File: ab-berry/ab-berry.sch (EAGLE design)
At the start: 27 parts, among them U1 LM1117MPX-3.3/NOPB or AP2114H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

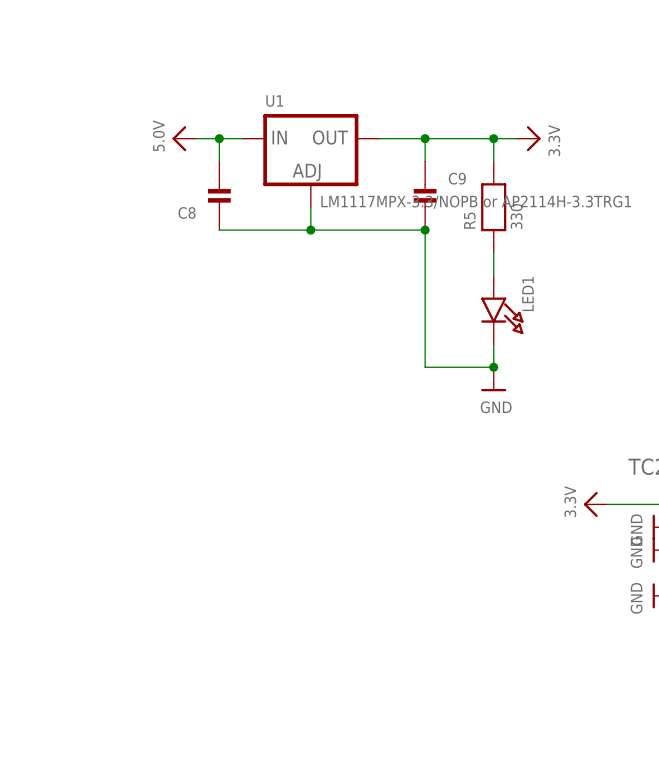
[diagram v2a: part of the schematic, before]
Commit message: wip
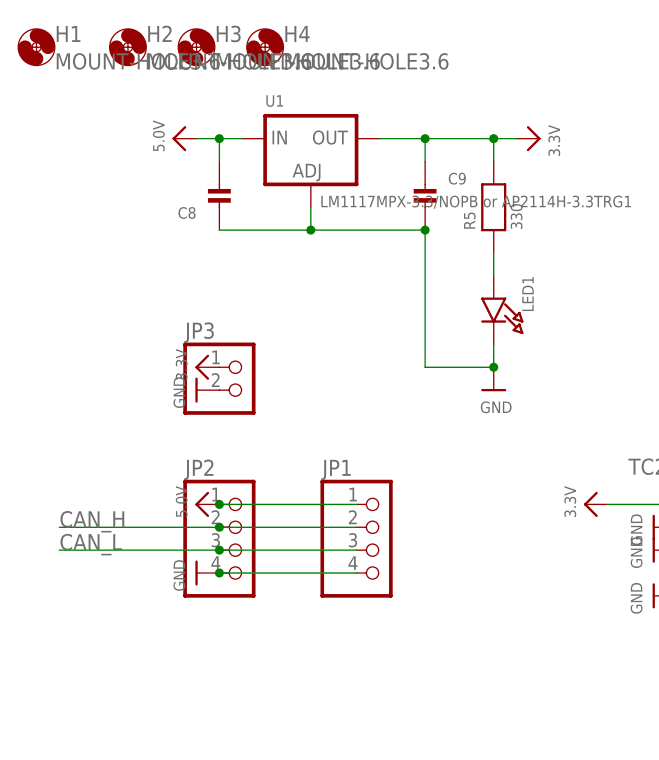
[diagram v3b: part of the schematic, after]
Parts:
- added H1, H2, H3, H4: MOUNT-HOLE3.6, holes:MOUNT-HOLE3.6
- added JP1, JP2: (no value), keves:PINHD-1X4
- added JP3: (no value), pinhead:PINHD-1X2
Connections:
- net 3.3V: now also JP3.1
- net 5.0V: now also JP1.1, JP2.1
- net CAN_H: now also JP1.2, JP2.2
- net CAN_L: now also JP1.3, JP2.3
- net GND: now also JP1.4, JP2.4, JP3.2
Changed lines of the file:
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@@
 <part name="U$27" library="microbuilder" deviceset="GND" device=""/>
 <part name="U$28" library="microbuilder" deviceset="3.3V" device=""/>
+<part name="JP1" library="keves" deviceset="PINHD-1X4" device=""/>
+<part name="JP2" library="keves" deviceset="PINHD-1X4" device=""/>
+<part name="U$30" library="microbuilder" deviceset="GND" device=""/>
+<part name="H1" library="holes" deviceset="MOUNT-HOLE" device="3.6"/>
+<part name="H2" library="holes" deviceset="MOUNT-HOLE" device="3.6"/>
+<part name="H3" library="holes" deviceset="MOUNT-HOLE" device="3.6"/>
+<part name="H4" library="holes" deviceset="MOUNT-HOLE" device="3.6"/>
+<part name="U$29" library="microbuilder" deviceset="5.0V" device=""/>
+<part name="JP3" library="pinhead" deviceset="PINHD-1X2" device=""/>
+<part name="U$31" library="microbuilder" deviceset="3.3V" device=""/>
+<part name="U$32" library="microbuilder" deviceset="GND" device=""/>
 </parts>
 <sheets>
@@
 <instance part="U$27" gate="G$1" x="109.22" y="-53.34" rot="R270"/>
 <instance part="U$28" gate="G$1" x="109.22" y="-50.8" rot="R90"/>
+<instance part="JP1" gate="A" x="-50.8" y="38.1"/>
+<instance part="JP2" gate="A" x="-66.04" y="38.1"/>
+<instance part="U$30" gate="G$1" x="-71.12" y="35.56" rot="R270"/>
+<instance part="H1" gate="G$1" x="-88.9" y="93.98"/>
+<instance part="H2" gate="G$1" x="-78.74" y="93.98"/>
+<instance part="H3" gate="G$1" x="-71.12" y="93.98"/>
+<instance part="H4" gate="G$1" x="-63.5" y="93.98"/>
+<instance part="U$29" gate="G$1" x="-71.12" y="43.18" rot="R90"/>
+<instance part="JP3" gate="G$1" x="-66.04" y="55.88"/>
+<instance part="U$31" gate="G$1" x="-71.12" y="58.42" rot="R90"/>
+<instance part="U$32" gate="G$1" x="-71.12" y="55.88" rot="R270"/>
 </instances>
 <busses>
@@
 <pinref part="LCD2" gate="G$1" pin="GND"/>
 <pinref part="U$27" gate="G$1" pin="GND"/>
+</segment>
+<segment>
+<pinref part="JP1" gate="A" pin="4"/>
+<pinref part="JP2" gate="A" pin="4"/>
+<wire x1="-68.58" y1="35.56" x2="-53.34" y2="35.56" width="0.1524" layer="91"/>
+<pinref part="U$30" gate="G$1" pin="GND"/>
+<junction x="-68.58" y="35.56"/>
+</segment>
+<segment>
+<pinref part="JP3" gate="G$1" pin="2"/>
+<pinref part="U$32" gate="G$1" pin="GND"/>
 </segment>
 </net>
@@
 <junction x="111.76" y="-50.8"/>
 </segment>
+<segment>
+<pinref part="JP3" gate="G$1" pin="1"/>
+<pinref part="U$31" gate="G$1" pin="3.3V"/>
+</segment>
 </net>
 <net name="SWDIO" class="0">
@@
 <label x="55.88" y="-22.86" size="1.778" layer="95"/>
 </segment>
+<segment>
+<pinref part="JP1" gate="A" pin="2"/>
+<pinref part="JP2" gate="A" pin="2"/>
+<wire x1="-68.58" y1="40.64" x2="-53.34" y2="40.64" width="0.1524" layer="91"/>
+<wire x1="-68.58" y1="40.64" x2="-86.36" y2="40.64" width="0.1524" layer="91"/>
+<junction x="-68.58" y="40.64"/>
+<label x="-86.36" y="40.64" size="1.778" layer="95"/>
+</segment>
 </net>
 <net name="CAN_L" class="0">
@@
 <wire x1="50.8" y1="-27.94" x2="58.42" y2="-27.94" width="0.1524" layer="91"/>
 <label x="55.88" y="-27.94" size="1.778" layer="95"/>
+</segment>
+<segment>
+<pinref part="JP1" gate="A" pin="3"/>
+<pinref part="JP2" gate="A" pin="3"/>
+<wire x1="-68.58" y1="38.1" x2="-53.34" y2="38.1" width="0.1524" layer="91"/>
+<wire x1="-68.58" y1="38.1" x2="-86.36" y2="38.1" width="0.1524" layer="91"/>
+<junction x="-68.58" y="38.1"/>
+<label x="-86.36" y="38.1" size="1.778" layer="95"/>
 </segment>
 </net>
@@
 <junction x="-68.58" y="83.82"/>
 </segment>
-</net>
+<segment>
+<pinref part="JP1" gate="A" pin="1"/>
+<pinref part="JP2" gate="A" pin="1"/>
+<wire x1="-68.58" y1="43.18" x2="-53.34" y2="43.18" width="0.1524" layer="91"/>
+<pinref part="U$29" gate="G$1" pin="5.0V"/>
+<junction x="-68.58" y="43.18"/>
+</segment>
+</net>

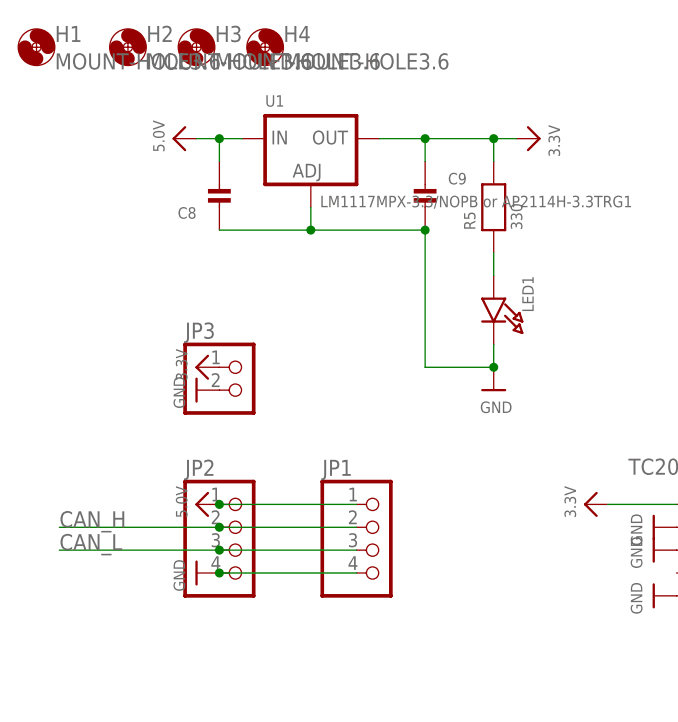
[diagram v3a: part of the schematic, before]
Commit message: wip
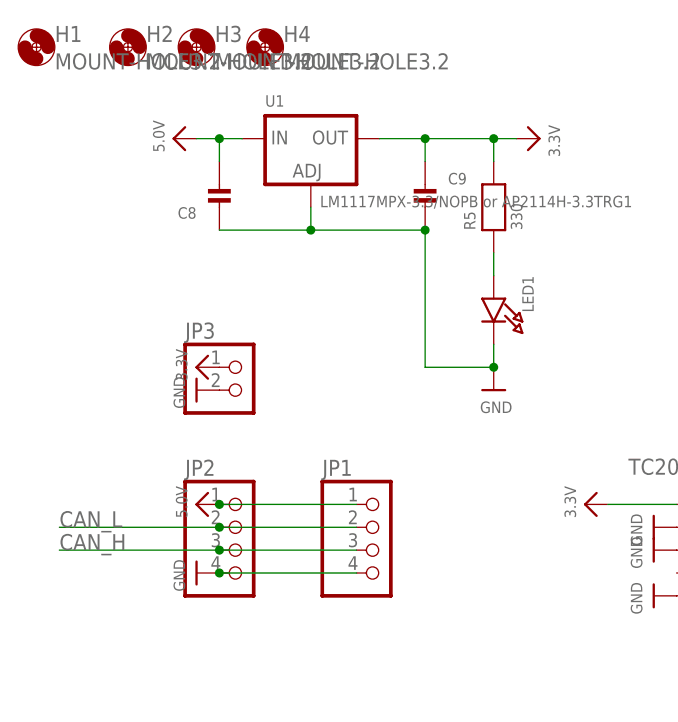
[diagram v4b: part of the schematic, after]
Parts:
- H1, H2, H3, H4: value MOUNT-HOLE3.6 -> MOUNT-HOLE3.2; device holes:MOUNT-HOLE3.6 -> holes:MOUNT-HOLE3.2
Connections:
- net CAN_H: now also JP1.3, JP2.3; no longer JP1.2, JP2.2
- net CAN_L: now also JP1.2, JP2.2; no longer JP1.3, JP2.3
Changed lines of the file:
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@@
 <grid distance="0.1" unitdist="inch" unit="inch" style="lines" multiple="1" display="no" altdistance="0.01" altunitdist="inch" altunit="inch"/>
 <layers>
-<layer number="1" name="Top" color="4" fill="1" visible="no" active="no"/>
-<layer number="16" name="Bottom" color="1" fill="1" visible="no" active="no"/>
-<layer number="17" name="Pads" color="2" fill="1" visible="no" active="no"/>
-<layer number="18" name="Vias" color="2" fill="1" visible="no" active="no"/>
-<layer number="19" name="Unrouted" color="6" fill="1" visible="no" active="no"/>
-<layer number="20" name="Dimension" color="15" fill="1" visible="no" active="no"/>
-<layer number="21" name="tPlace" color="7" fill="1" visible="no" active="no"/>
-<layer number="22" name="bPlace" color="7" fill="1" visible="no" active="no"/>
-<layer number="23" name="tOrigins" color="15" fill="1" visible="no" active="no"/>
-<layer number="24" name="bOrigins" color="15" fill="1" visible="no" active="no"/>
-<layer number="25" name="tNames" color="7" fill="1" visible="no" active="no"/>
-<layer number="26" name="bNames" color="7" fill="1" visible="no" active="no"/>
-<layer number="27" name="tValues" color="7" fill="1" visible="no" active="no"/>
-<layer number="28" name="bValues" color="7" fill="1" visible="no" active="no"/>
+<layer number="1" name="Top" color="4" fill="1" visible="yes" active="no"/>
+<layer number="16" name="Bottom" color="1" fill="1" visible="yes" active="no"/>
+<layer number="17" name="Pads" color="2" fill="1" visible="yes" active="no"/>
+<layer number="18" name="Vias" color="2" fill="1" visible="yes" active="no"/>
+<layer number="19" name="Unrouted" color="6" fill="1" visible="yes" active="no"/>
+<layer number="20" name="Dimension" color="15" fill="1" visible="yes" active="no"/>
+<layer number="21" name="tPlace" color="7" fill="1" visible="yes" active="no"/>
+<layer number="22" name="bPlace" color="7" fill="1" visible="yes" active="no"/>
+<layer number="23" name="tOrigins" color="15" fill="1" visible="yes" active="no"/>
+<layer number="24" name="bOrigins" color="15" fill="1" visible="yes" active="no"/>
+<layer number="25" name="tNames" color="7" fill="1" visible="yes" active="no"/>
+<layer number="26" name="bNames" color="7" fill="1" visible="yes" active="no"/>
+<layer number="27" name="tValues" color="7" fill="1" visible="yes" active="no"/>
+<layer number="28" name="bValues" color="7" fill="1" visible="yes" active="no"/>
 <layer number="29" name="tStop" color="7" fill="3" visible="no" active="no"/>
 <layer number="30" name="bStop" color="7" fill="6" visible="no" active="no"/>
@@
 <layer number="35" name="tGlue" color="7" fill="4" visible="no" active="no"/>
 <layer number="36" name="bGlue" color="7" fill="5" visible="no" active="no"/>
-<layer number="37" name="tTest" color="7" fill="1" visible="no" active="no"/>
-<layer number="38" name="bTest" color="7" fill="1" visible="no" active="no"/>
+<layer number="37" name="tTest" color="7" fill="1" visible="yes" active="no"/>
+<layer number="38" name="bTest" color="7" fill="1" visible="yes" active="no"/>
 <layer number="39" name="tKeepout" color="4" fill="11" visible="no" active="no"/>
 <layer number="40" name="bKeepout" color="1" fill="11" visible="no" active="no"/>
@@
 <layer number="44" name="Drills" color="7" fill="1" visible="no" active="no"/>
 <layer number="45" name="Holes" color="7" fill="1" visible="no" active="no"/>
-<layer number="46" name="Milling" color="3" fill="1" visible="no" active="no"/>
-<layer number="47" name="Measures" color="7" fill="1" visible="no" active="no"/>
-<layer number="48" name="Document" color="7" fill="1" visible="no" active="no"/>
-<layer number="49" name="Reference" color="7" fill="1" visible="no" active="no"/>
-<layer number="50" name="dxf" color="7" fill="1" visible="no" active="no"/>
-<layer number="51" name="tDocu" color="7" fill="1" visible="no" active="no"/>
-<layer number="52" name="bDocu" color="7" fill="1" visible="no" active="no"/>
-<layer number="53" name="tGND_GNDA" color="7" fill="9" visible="no" active="no"/>
-<layer number="54" name="bGND_GNDA" color="1" fill="9" visible="no" active="no"/>
-<layer number="56" name="wert" color="7" fill="1" visible="no" active="no"/>
+<layer number="46" name="Milling" color="3" fill="1" visible="yes" active="no"/>
+<layer number="47" name="Measures" color="7" fill="1" visible="yes" active="no"/>
+<layer number="48" name="Document" color="7" fill="1" visible="yes" active="no"/>
+<layer number="49" name="Reference" color="7" fill="1" visible="yes" active="no"/>
+<layer number="50" name="dxf" color="7" fill="1" visible="yes" active="no"/>
+<layer number="51" name="tDocu" color="7" fill="1" visible="yes" active="no"/>
+<layer number="52" name="bDocu" color="7" fill="1" visible="yes" active="no"/>
+<layer number="53" name="tGND_GNDA" color="7" fill="9" visible="yes" active="no"/>
+<layer number="54" name="bGND_GNDA" color="1" fill="9" visible="yes" active="no"/>
+<layer number="56" name="wert" color="7" fill="1" visible="yes" active="no"/>
 <layer number="90" name="Modules" color="5" fill="1" visible="yes" active="yes"/>
 <layer number="91" name="Nets" color="2" fill="1" visible="yes" active="yes"/>
@@
 <part name="JP2" library="keves" deviceset="PINHD-1X4" device=""/>
 <part name="U$30" library="microbuilder" deviceset="GND" device=""/>
-<part name="H1" library="holes" deviceset="MOUNT-HOLE" device="3.6"/>
-<part name="H2" library="holes" deviceset="MOUNT-HOLE" device="3.6"/>
-<part name="H3" library="holes" deviceset="MOUNT-HOLE" device="3.6"/>
-<part name="H4" library="holes" deviceset="MOUNT-HOLE" device="3.6"/>
+<part name="H1" library="holes" deviceset="MOUNT-HOLE" device="3.2" value="MOUNT-HOLE3.2"/>
+<part name="H2" library="holes" deviceset="MOUNT-HOLE" device="3.2" value="MOUNT-HOLE3.2"/>
+<part name="H3" library="holes" deviceset="MOUNT-HOLE" device="3.2" value="MOUNT-HOLE3.2"/>
+<part name="H4" library="holes" deviceset="MOUNT-HOLE" device="3.2" value="MOUNT-HOLE3.2"/>
 <part name="U$29" library="microbuilder" deviceset="5.0V" device=""/>
 <part name="JP3" library="pinhead" deviceset="PINHD-1X2" device=""/>
@@
 </segment>
 <segment>
+<pinref part="JP1" gate="A" pin="3"/>
+<pinref part="JP2" gate="A" pin="3"/>
+<wire x1="-68.58" y1="38.1" x2="-53.34" y2="38.1" width="0.1524" layer="91"/>
+<wire x1="-68.58" y1="38.1" x2="-86.36" y2="38.1" width="0.1524" layer="91"/>
+<junction x="-68.58" y="38.1"/>
+<label x="-86.36" y="38.1" size="1.778" layer="95"/>
+</segment>
+</net>
+<net name="CAN_L" class="0">
+<segment>
+<pinref part="D1" gate="G$1" pin="CANL"/>
+<wire x1="50.8" y1="-27.94" x2="58.42" y2="-27.94" width="0.1524" layer="91"/>
+<label x="55.88" y="-27.94" size="1.778" layer="95"/>
+</segment>
+<segment>
 <pinref part="JP1" gate="A" pin="2"/>
 <pinref part="JP2" gate="A" pin="2"/>
@@
 </segment>
 </net>
-<net name="CAN_L" class="0">
-<segment>
-<pinref part="D1" gate="G$1" pin="CANL"/>
-<wire x1="50.8" y1="-27.94" x2="58.42" y2="-27.94" width="0.1524" layer="91"/>
-<label x="55.88" y="-27.94" size="1.778" layer="95"/>
-</segment>
-<segment>
-<pinref part="JP1" gate="A" pin="3"/>
-<pinref part="JP2" gate="A" pin="3"/>
-<wire x1="-68.58" y1="38.1" x2="-53.34" y2="38.1" width="0.1524" layer="91"/>
-<wire x1="-68.58" y1="38.1" x2="-86.36" y2="38.1" width="0.1524" layer="91"/>
-<junction x="-68.58" y="38.1"/>
-<label x="-86.36" y="38.1" size="1.778" layer="95"/>
-</segment>
-</net>
